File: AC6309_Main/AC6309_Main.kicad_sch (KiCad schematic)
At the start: 18 parts, among them J1 Address, J2 Data and Control, SW1 Reset, U1 HD63B09P, U2 W24257, U3 28C256, U4 MC68B50, U5 74HCT00, U6 74HC138, Y1 7.3728 MHz

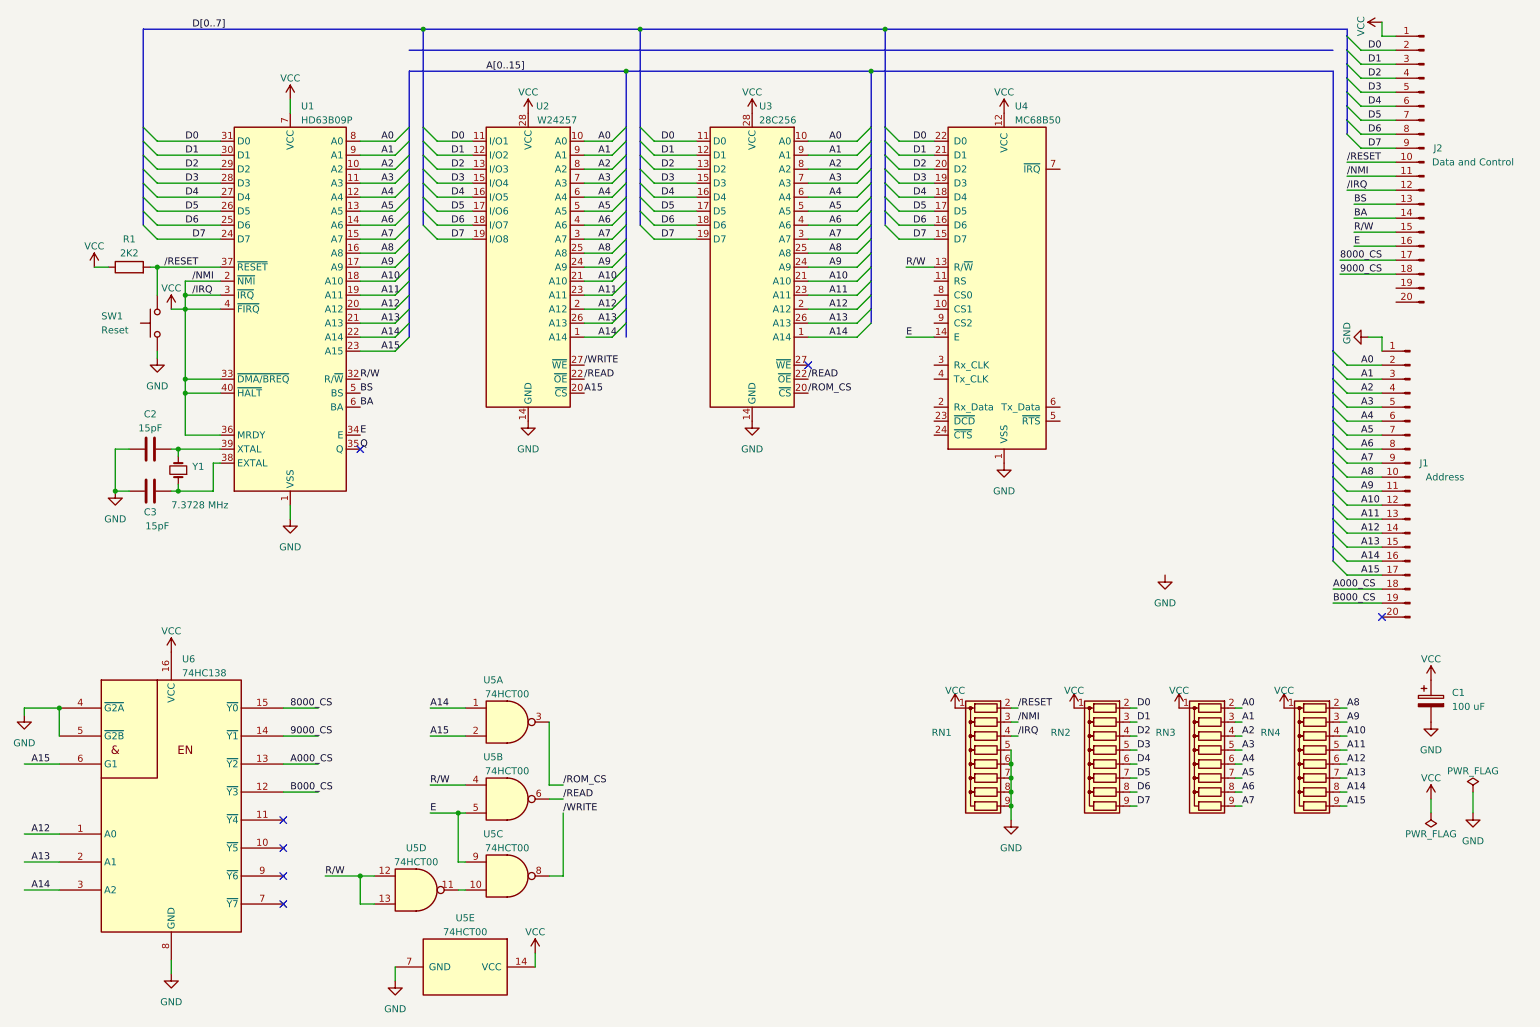
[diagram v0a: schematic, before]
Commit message: Schematics revision 1, Digital file, etc.
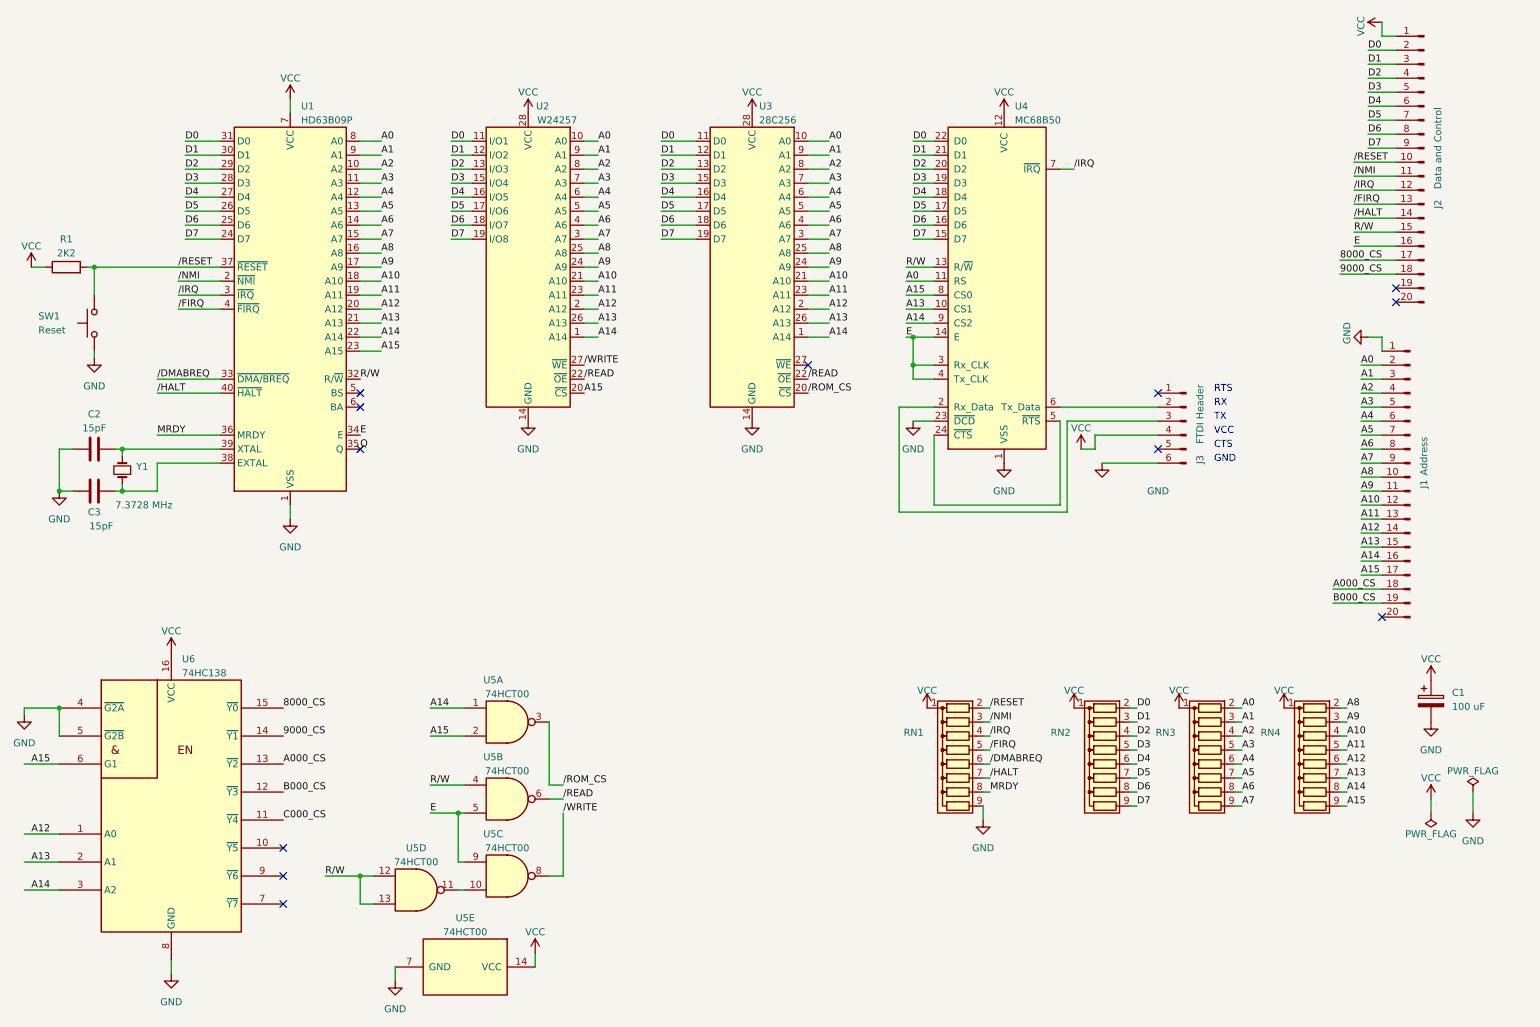
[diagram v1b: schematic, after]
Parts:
- added J3: FTDI Header, Connector_PinHeader_2.54mm:PinHeader_1x06_P2.54mm_Vertical, symbol Connector:Conn_01x06_Pin
- J1, J2: footprint Connector_PinHeader_2.00mm:PinHeader_1x20_P2.00mm_Vertical -> Connector_PinHeader_2.54mm:PinHeader_1x20_P2.54mm_Vertical
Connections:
- net A0: now also U4.11 (RS)
- net A13: now also U4.10 (CS1)
- net A14: now also U4.9 (CS2)
- net A15: now also U4.8 (CS0)
- net E: now also U4.3 (Rx_CLK), U4.4 (Tx_CLK)
- net GND: now also U4.23 (~{DCD}), J3.6 (Pin_6); no longer RN1.5 (R4), RN1.6 (R5), RN1.7 (R6), RN1.8 (R7)
- net VCC: now also J3.4 (Pin_4); no longer J2.11 (Pin_11), J2.12 (Pin_12), RN1.3 (R2), RN1.4 (R3), U1.2 (~{NMI}), U1.3 (~{IRQ}), U1.33 (~{DMA/BREQ}), U1.36 (MRDY), U1.4 (~{FIRQ}), U1.40 (~{HALT})
- net C000_CS: now reaches U6.11 (~{Y4})
- net at U4.2 (Rx_Data): now also J3.3 (Pin_3)
- net at U4.24 (~{CTS}): now also U4.5 (~{RTS})
- net at U4.6 (Tx_Data): now also J3.2 (Pin_2)
- net /IRQ: now reaches U4.7 (~{IRQ})
- net /IRQ: now also J2.12 (Pin_12), RN1.4 (R3), U1.3 (~{IRQ})
- net BA: no longer names the net of U1.6 (BA)
- net BA: no longer J2.14 (Pin_14)
- net BS: no longer names the net of U1.5 (BS)
- net BS: no longer J2.13 (Pin_13)
- new net MRDY: RN1.8 (R7), U1.36 (MRDY)
- new net /DMABREQ: RN1.6 (R5), U1.33 (~{DMA/BREQ})
- new net /FIRQ: J2.13 (Pin_13), RN1.5 (R4), U1.4 (~{FIRQ})
- new net /HALT: J2.14 (Pin_14), RN1.7 (R6), U1.40 (~{HALT})
- new net /NMI: J2.11 (Pin_11), RN1.3 (R2), U1.2 (~{NMI})
- no-connect marks 7 -> 12
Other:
- note added: "CTS"
- note added: "GND"
- note added: "RTS"
- note added: "RX"
- note added: "TX"
- note added: "VCC"
- moved on the sheet: C2, C3, R1, RN1, SW1, Y1
